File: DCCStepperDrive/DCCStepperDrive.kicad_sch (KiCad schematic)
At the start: 32 parts, among them J1 12v, J2 CBUS, J3 5V select, J4 DCC, J5 Grove 2mm, J6 I2C, J7 Sensor, J8 Motor, J9 Mode Select, Q1 DMG2305UX-7, SW1 SW_Push, U1 AMS1117-3.3, U2 AMS1117-5.0, U3 6N137, U4 Pico

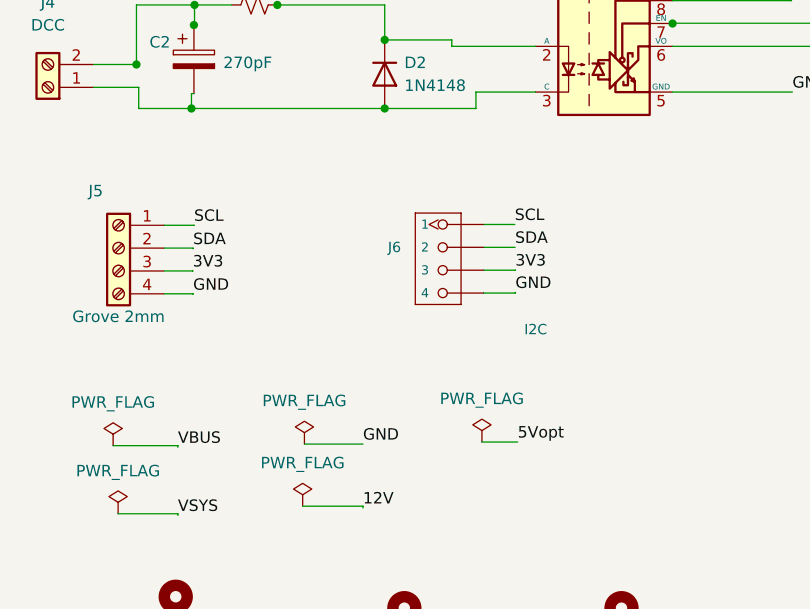
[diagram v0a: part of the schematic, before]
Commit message: 21:25 Titan.local
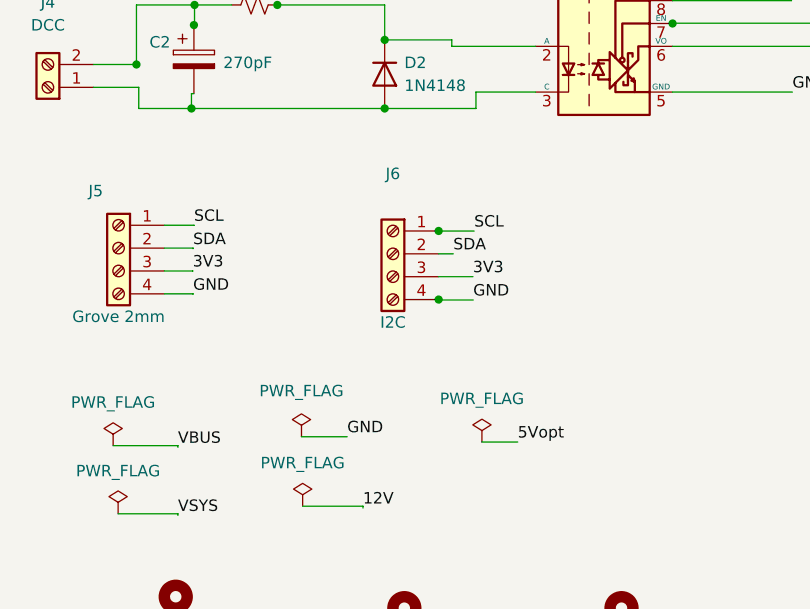
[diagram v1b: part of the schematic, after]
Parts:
- removed J6: I2C, OPL_Connector:HW4-2.0, symbol OPL_Connector:GROVE-CONNECTOR-DIP_4P-2.0_
- added J6: I2C, OPL_Connector:HW4-2.0, symbol Connector:Screw_Terminal_01x04
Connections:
- net 3V3: now also J6.3 (Pin_3)
- net GND: now also J6.4 (Pin_4)
- net SCL: now also J6.1 (Pin_1)
- net SDA: now also J6.2 (Pin_2)
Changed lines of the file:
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@@
   (junction (at 58.777 126.09) (diameter 0) (color 0 0 0 0)
   )
+  (junction (at 64.77 147.32) (diameter 0) (color 0 0 0 0)
+  )
   (junction (at 31.1947 128.8215) (diameter 0) (color 0 0 0 0)
   )
@@
   )
   (junction (at 145.1614 59.6484) (diameter 0) (color 0 0 0 0)
+  )
+  (junction (at 64.77 154.94) (diameter 0) (color 0 0 0 0)
   )
   (junction (at 121.3322 23.5497) (diameter 0) (color 0 0 0 0)
@@
     (stroke (width 0) (type default) (color 0 0 0 0))
   )
+  (wire (pts (xy 68.6141 154.987) (xy 64.77 154.987))
+    (stroke (width 0) (type default) (color 0 0 0 0))
+  )
   (wire (pts (xy 29.158 178.7396) (xy 35.8026 178.7396))
     (stroke (width 0) (type default) (color 0 0 0 0))
@@
     (stroke (width 0) (type default) (color 0 0 0 0))
   )
+  (wire (pts (xy 64.77 147.3282) (xy 64.77 147.32))
+    (stroke (width 0) (type default) (color 0 0 0 0))
+  )
   (wire (pts (xy 198.9334 52.1418) (xy 180.7214 52.1418))
     (stroke (width 0) (type default) (color 0 0 0 0))
@@
     (stroke (width 0) (type default) (color 0 0 0 0))
   )
+  (wire (pts (xy 49.53 170.18) (xy 54.61 170.18))
+    (stroke (width 0) (type default) (color 0 0 0 0))
+  )
   (wire (pts (xy 117.1897 136.3294) (xy 117.1897 136.4986))
     (stroke (width 0) (type default) (color 0 0 0 0))
@@
     (stroke (width 0) (type default) (color 0 0 0 0))
   )
+  (wire (pts (xy 68.7162 147.3282) (xy 64.77 147.3282))
+    (stroke (width 0) (type default) (color 0 0 0 0))
+  )
   (wire (pts (xy 91.5231 25.1346) (xy 96.7551 25.1346))
     (stroke (width 0) (type default) (color 0 0 0 0))
@@
     (stroke (width 0) (type default) (color 0 0 0 0))
   )
-  (wire (pts (xy 69.7981 154.2174) (xy 73.2984 154.2174))
-    (stroke (width 0) (type default) (color 0 0 0 0))
-  )
   (wire (pts (xy 91.7448 52.3853) (xy 91.7448 52.4764))
     (stroke (width 0) (type default) (color 0 0 0 0))
@@
     (stroke (width 0) (type default) (color 0 0 0 0))
   )
+  (wire (pts (xy 66.3965 149.86) (xy 64.77 149.86))
+    (stroke (width 0) (type default) (color 0 0 0 0))
+  )
+  (wire (pts (xy 64.77 154.987) (xy 64.77 154.94))
+    (stroke (width 0) (type default) (color 0 0 0 0))
+  )
   (wire (pts (xy 111.514 59.6484) (xy 122.9589 59.6484))
     (stroke (width 0) (type default) (color 0 0 0 0))
@@
     (stroke (width 0) (type default) (color 0 0 0 0))
   )
-  (wire (pts (xy 73.2984 151.6774) (xy 73.2984 151.6606))
-    (stroke (width 0) (type default) (color 0 0 0 0))
-  )
   (wire (pts (xy 245.11 22.225) (xy 247.65 22.225))
     (stroke (width 0) (type default) (color 0 0 0 0))
@@
     (stroke (width 0) (type default) (color 0 0 0 0))
   )
-  (wire (pts (xy 69.7981 146.5974) (xy 73.2303 146.5974))
-    (stroke (width 0) (type default) (color 0 0 0 0))
-  )
   (wire (pts (xy 58.42 52.2923) (xy 62.8797 52.2923))
     (stroke (width 0) (type default) (color 0 0 0 0))
@@
     (stroke (width 0) (type default) (color 0 0 0 0))
   )
-  (wire (pts (xy 69.7981 151.6774) (xy 73.2984 151.6774))
-    (stroke (width 0) (type default) (color 0 0 0 0))
-  )
   (wire (pts (xy 266.8544 62.23) (xy 266.8544 61.976))
     (stroke (width 0) (type default) (color 0 0 0 0))
@@
     (stroke (width 0) (type default) (color 0 0 0 0))
   )
-  (wire (pts (xy 49.8592 171.0002) (xy 56.3645 171.0002))
-    (stroke (width 0) (type default) (color 0 0 0 0))
-  )
   (wire (pts (xy 224.79 46.99) (xy 224.79 38.735))
     (stroke (width 0) (type default) (color 0 0 0 0))
@@
     (stroke (width 0) (type default) (color 0 0 0 0))
   )
-  (wire (pts (xy 69.7981 149.1374) (xy 73.2643 149.1374))
-    (stroke (width 0) (type default) (color 0 0 0 0))
-  )
   (wire (pts (xy 234.95 44.7196) (xy 234.95 46.99))
     (stroke (width 0) (type default) (color 0 0 0 0))
@@
     (stroke (width 0) (type default) (color 0 0 0 0))
   )
-  (wire (pts (xy 73.2984 154.2174) (xy 73.2984 154.1455))
-    (stroke (width 0) (type default) (color 0 0 0 0))
-  )
   (wire (pts (xy 247.65 46.99) (xy 247.65 43.815))
     (stroke (width 0) (type default) (color 0 0 0 0))
@@
     (stroke (width 0) (type default) (color 0 0 0 0))
   )
+  (wire (pts (xy 64.77 152.4) (xy 68.58 152.4))
+    (stroke (width 0) (type default) (color 0 0 0 0))
+  )
   (wire (pts (xy 128.0486 126.9774) (xy 128.0486 126.9603))
     (stroke (width 0) (type default) (color 0 0 0 0))
@@
   )
   (label "VBUS" (at 34.29 73.66 0)
+    (effects (font (size 1.27 1.27)) (justify left bottom))
+  )
+  (label "SCL" (at 68.7162 147.3282 0)
     (effects (font (size 1.27 1.27)) (justify left bottom))
   )
@@
     (effects (font (size 1.27 1.27)) (justify right bottom))
   )
-  (label "3V3" (at 73.2984 151.6606 0)
-    (effects (font (size 1.27 1.27)) (justify left bottom))
-  )
   (label "GND" (at 104.0798 131.8857 0)
     (effects (font (size 1.27 1.27)) (justify left bottom))
@@
     (effects (font (size 1.27 1.27)) (justify left bottom))
   )
+  (label "GND" (at 68.6141 154.987 0)
+    (effects (font (size 1.27 1.27)) (justify left bottom))
+  )
   (label "VBUS" (at 35.8026 171.3567 0)
     (effects (font (size 1.27 1.27)) (justify left bottom))
   )
-  (label "SCL" (at 73.2303 146.5974 0)
-    (effects (font (size 1.27 1.27)) (justify left bottom))
-  )
   (label "GND" (at 185.1197 80.0791 0)
     (effects (font (size 1.27 1.27)) (justify left bottom))
@@
     (effects (font (size 1.27 1.27)) (justify left bottom))
   )
-  (label "GND" (at 56.3645 171.0002 0)
-    (effects (font (size 1.27 1.27)) (justify left bottom))
-  )
   (label "SDA" (at 190.6195 72.3977 0)
     (effects (font (size 1.27 1.27)) (justify left bottom))
   )
+  (label "3V3" (at 68.58 152.4 0)
+    (effects (font (size 1.27 1.27)) (justify left bottom))
+  )
   (label "GND" (at 37.4893 154.3497 0)
     (effects (font (size 1.27 1.27)) (justify left bottom))
   )
   (label "5Vopt" (at 21.3957 87.3496 0)
+    (effects (font (size 1.27 1.27)) (justify left bottom))
+  )
+  (label "GND" (at 54.61 170.18 0)
     (effects (font (size 1.27 1.27)) (justify left bottom))
   )
@@
     (effects (font (size 1.27 1.27)) (justify left bottom))
   )
+  (label "SDA" (at 66.3965 149.86 0)
+    (effects (font (size 1.27 1.27)) (justify left bottom))
+  )
   (label "SCL" (at 190.6588 127.1829 0)
     (effects (font (size 1.27 1.27)) (justify left bottom))
@@
   )
   (label "VBUS" (at 90.6042 60.3334 0)
-    (effects (font (size 1.27 1.27)) (justify left bottom))
-  )
-  (label "SDA" (at 73.2643 149.1374 0)
-    (effects (font (size 1.27 1.27)) (justify left bottom))
-  )
-  (label "GND" (at 73.2984 154.1455 0)
     (effects (font (size 1.27 1.27)) (justify left bottom))
   )
@@
       (effects (font (size 1.27 1.27)) hide)
     )
+  )
+  (symbol (lib_id "Connector:Screw_Terminal_01x04") (at 59.69 149.86 0) (mirror y) (unit 1)
+    (in_bom yes) (on_board yes)
+    (property "Reference" "J6" (id 0) (at 59.69 140.97 0))
+    (property "Value" "I2C" (id 1) (at 59.69 157.48 0))
+    (property "Footprint" "OPL_Connector:HW4-2.0" (id 2) (at 59.69 149.86 0)
+      (effects (font (size 1.27 1.27)) hide)
+    )
+    (property "Datasheet" "~" (id 3) (at 59.69 149.86 0)
+      (effects (font (size 1.27 1.27)) hide)
+    )
+    (pin "1")
+    (pin "2")
+    (pin "3")
+    (pin "4")
   )
   (symbol (lib_id "Diode:1N4148") (at 58.777 129.9 270) (unit 1)
@@
     (pin "8")
   )
-  (symbol (lib_id "OPL_Connector:GROVE-CONNECTOR-DIP_4P-2.0_") (at 65.9881 150.4074 0) (mirror y) (unit 1)
-    (in_bom yes) (on_board yes)
-    (property "Reference" "J6" (id 0) (at 60.5938 149.1374 0)
-      (effects (font (size 1.143 1.143)) (justify left))
-    )
-    (property "Value" "I2C" (id 1) (at 76.8277 158.2627 0)
-      (effects (font (size 1.143 1.143)) (justify left))
-    )
-    (property "Footprint" "OPL_Connector:HW4-2.0" (id 2) (at 65.9881 150.4074 0)
-      (effects (font (size 1.27 1.27)) hide)
-    )
-    (property "Datasheet" "" (id 3) (at 65.9881 150.4074 0)
-      (effects (font (size 1.27 1.27)) hide)
-    )
-    (property "SKU" "320110033" (id 4) (at 65.2261 146.5974 0)
-      (effects (font (size 0.508 0.508)) hide)
-    )
-    (pin "1")
-    (pin "2")
-    (pin "3")
-    (pin "4")
-  )
-  (symbol (lib_id "power:PWR_FLAG") (at 49.8592 171.0002 0) (unit 1)
-    (in_bom yes) (on_board yes) (fields_autoplaced)
-    (property "Reference" "#FLG04" (id 0) (at 49.8592 169.0952 0)
-      (effects (font (size 1.27 1.27)) hide)
-    )
-    (property "Value" "PWR_FLAG" (id 1) (at 49.8592 166.198 0))
-    (property "Footprint" "" (id 2) (at 49.8592 171.0002 0)
-      (effects (font (size 1.27 1.27)) hide)
-    )
-    (property "Datasheet" "~" (id 3) (at 49.8592 171.0002 0)
-      (effects (font (size 1.27 1.27)) hide)
-    )
-    (pin "1")
-  )
   (symbol (lib_id "Switch:SW_Push") (at 128.0389 59.646 0) (unit 1)
     (in_bom yes) (on_board yes)
@@
     (pin "4")
   )
+  (symbol (lib_id "power:PWR_FLAG") (at 49.53 170.18 0) (unit 1)
+    (in_bom yes) (on_board yes) (fields_autoplaced)
+    (property "Reference" "#FLG04" (id 0) (at 49.53 168.275 0)
+      (effects (font (size 1.27 1.27)) hide)
+    )
+    (property "Value" "PWR_FLAG" (id 1) (at 49.53 165.1 0))
+    (property "Footprint" "" (id 2) (at 49.53 170.18 0)
+      (effects (font (size 1.27 1.27)) hide)
+    )
+    (property "Datasheet" "~" (id 3) (at 49.53 170.18 0)
+      (effects (font (size 1.27 1.27)) hide)
+    )
+    (pin "1")
+  )
   (sheet_instances
     (path "/" (page "1"))
@@
       (reference "#FLG03") (unit 1) (value "PWR_FLAG") (footprint "")
     )
-    (path "/cbb3f860-16d5-4a0c-b263-c16249281626"
+    (path "/ffab892f-e249-418b-9af1-9dd6928db248"
       (reference "#FLG04") (unit 1) (value "PWR_FLAG") (footprint "")
     )
@@
       (reference "J5") (unit 1) (value "Grove 2mm") (footprint "OPL_Connector:HW4-2.0")
     )
-    (path "/cb567441-8070-43a6-91a4-d05496d8ca81"
+    (path "/8f809ce2-5e0c-4d4f-a5d1-5aaa77313ab2"
       (reference "J6") (unit 1) (value "I2C") (footprint "OPL_Connector:HW4-2.0")
     )

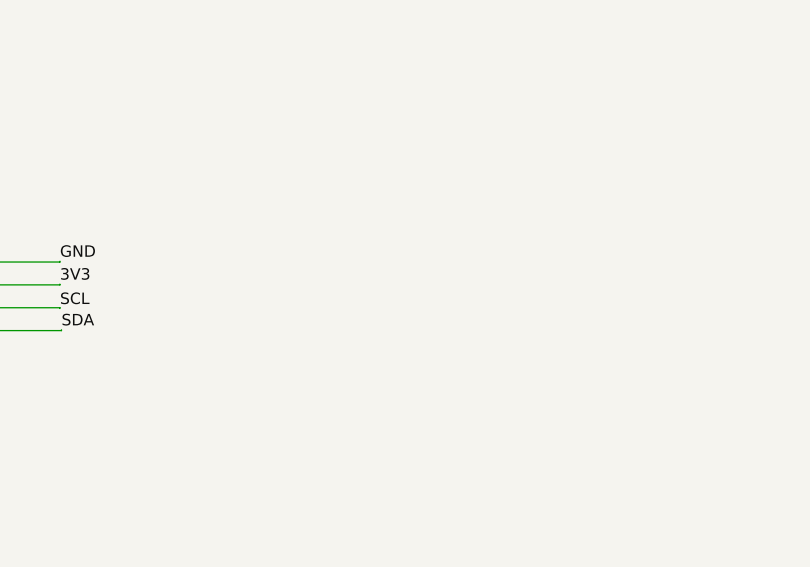
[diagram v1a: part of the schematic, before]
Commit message: 10:23 Arrakis.local
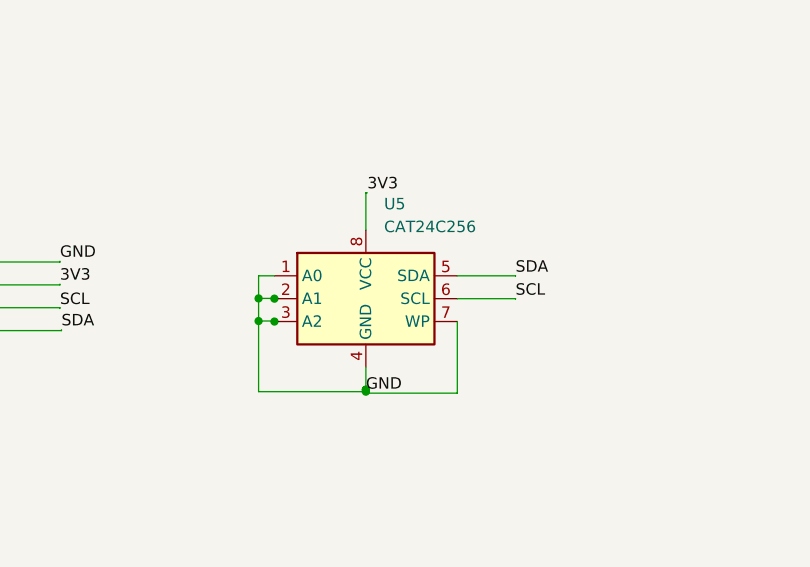
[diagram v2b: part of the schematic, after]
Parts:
- added U5: CAT24C256, Package_DIP:DIP-8_W7.62mm_LongPads, symbol Memory_EEPROM:CAT24C256
- R1, R2, R3, R4, R5: footprint Resistor_THT:R_Axial_DIN0207_L6.3mm_D2.5mm_P10.16mm_Horizontal -> Resistor_SMD:R_1206_3216Metric
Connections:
- net 3V3: now also U5.8 (VCC)
- net GND: now also U5.1 (A0), U5.2 (A1), U5.3 (A2), U5.4 (GND), U5.7 (WP)
- net SCL: now also U5.6 (SCL)
- net SDA: now also U5.5 (SDA)

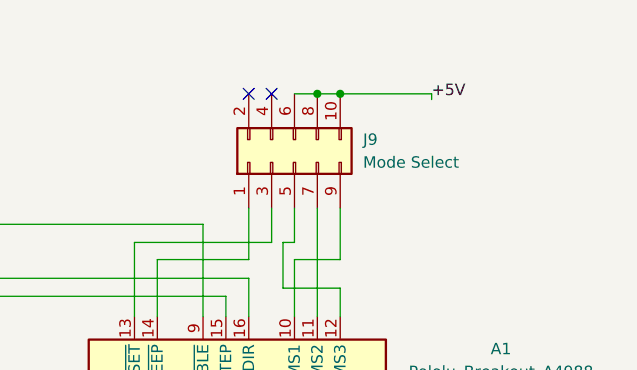
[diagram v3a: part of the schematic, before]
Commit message: 20:02 Arrakis.local
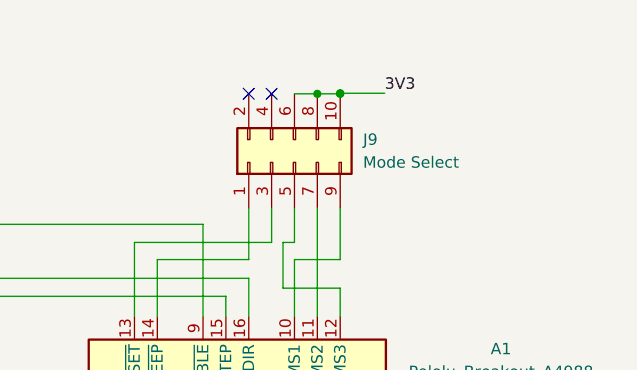
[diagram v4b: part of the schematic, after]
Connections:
- net +5V is gone; now on net 3V3: J9.10 (Pin_10), J9.6 (Pin_6), J9.8 (Pin_8)
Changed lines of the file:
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@@
     (comment 2 "2 Interface for sensor added")
     (comment 3 "3 Oled added")
+    (comment 4 "4 mode select on A4988 now to 3v3")
   )
   (junction (at 39.37 100.254) (diameter 0) (color 0 0 0 0)
@@
   )
   (junction (at 212.7293 126.0606) (diameter 0) (color 0 0 0 0)
+  )
+  (junction (at 247.65 22.1592) (diameter 0) (color 0 0 0 0)
   )
   (junction (at 128.0486 126.9603) (diameter 0) (color 0 0 0 0)
@@
     (stroke (width 0) (type default) (color 0 0 0 0))
   )
-  (wire (pts (xy 257.81 22.225) (xy 257.81 22.86))
-    (stroke (width 0) (type default) (color 0 0 0 0))
-  )
   (wire (pts (xy 192.4852 23.5497) (xy 121.3322 23.5497))
     (stroke (width 0) (type default) (color 0 0 0 0))
@@
     (stroke (width 0) (type default) (color 0 0 0 0))
   )
-  (wire (pts (xy 247.65 22.225) (xy 257.81 22.225))
-    (stroke (width 0) (type default) (color 0 0 0 0))
-  )
   (wire (pts (xy 145.1614 59.646) (xy 145.1614 59.6484))
     (stroke (width 0) (type default) (color 0 0 0 0))
@@
     (stroke (width 0) (type default) (color 0 0 0 0))
   )
+  (wire (pts (xy 247.65 22.1592) (xy 247.65 22.225))
+    (stroke (width 0) (type default) (color 0 0 0 0))
+  )
   (wire (pts (xy 242.57 22.225) (xy 245.11 22.225))
     (stroke (width 0) (type default) (color 0 0 0 0))
   )
+  (wire (pts (xy 252.6002 22.1592) (xy 247.65 22.1592))
+    (stroke (width 0) (type default) (color 0 0 0 0))
+  )
   (wire (pts (xy 43.1726 24.0152) (xy 42.4284 24.0044))
     (stroke (width 0) (type default) (color 0 0 0 0))
@@
   )
   (label "SCL" (at 68.7162 147.3282 0)
-    (effects (font (size 1.27 1.27)) (justify left bottom))
-  )
-  (label "+5V" (at 257.81 22.86 0)
     (effects (font (size 1.27 1.27)) (justify left bottom))
   )
@@
     (effects (font (size 1.27 1.27)) (justify left bottom))
   )
+  (label "3V3" (at 252.6002 22.1592 0)
+    (effects (font (size 1.27 1.27)) (justify left bottom))
+  )
